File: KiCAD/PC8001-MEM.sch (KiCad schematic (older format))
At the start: 37 parts, among them J1 PC-8001 ext BUS, U1 74LS32, U10 628128, U2 74LS138, U3 ULN2003A, U4 74LS138, U5 74LS175, U6 74LS32, U7 74LS541, U8 74LS273, U9 74LS541

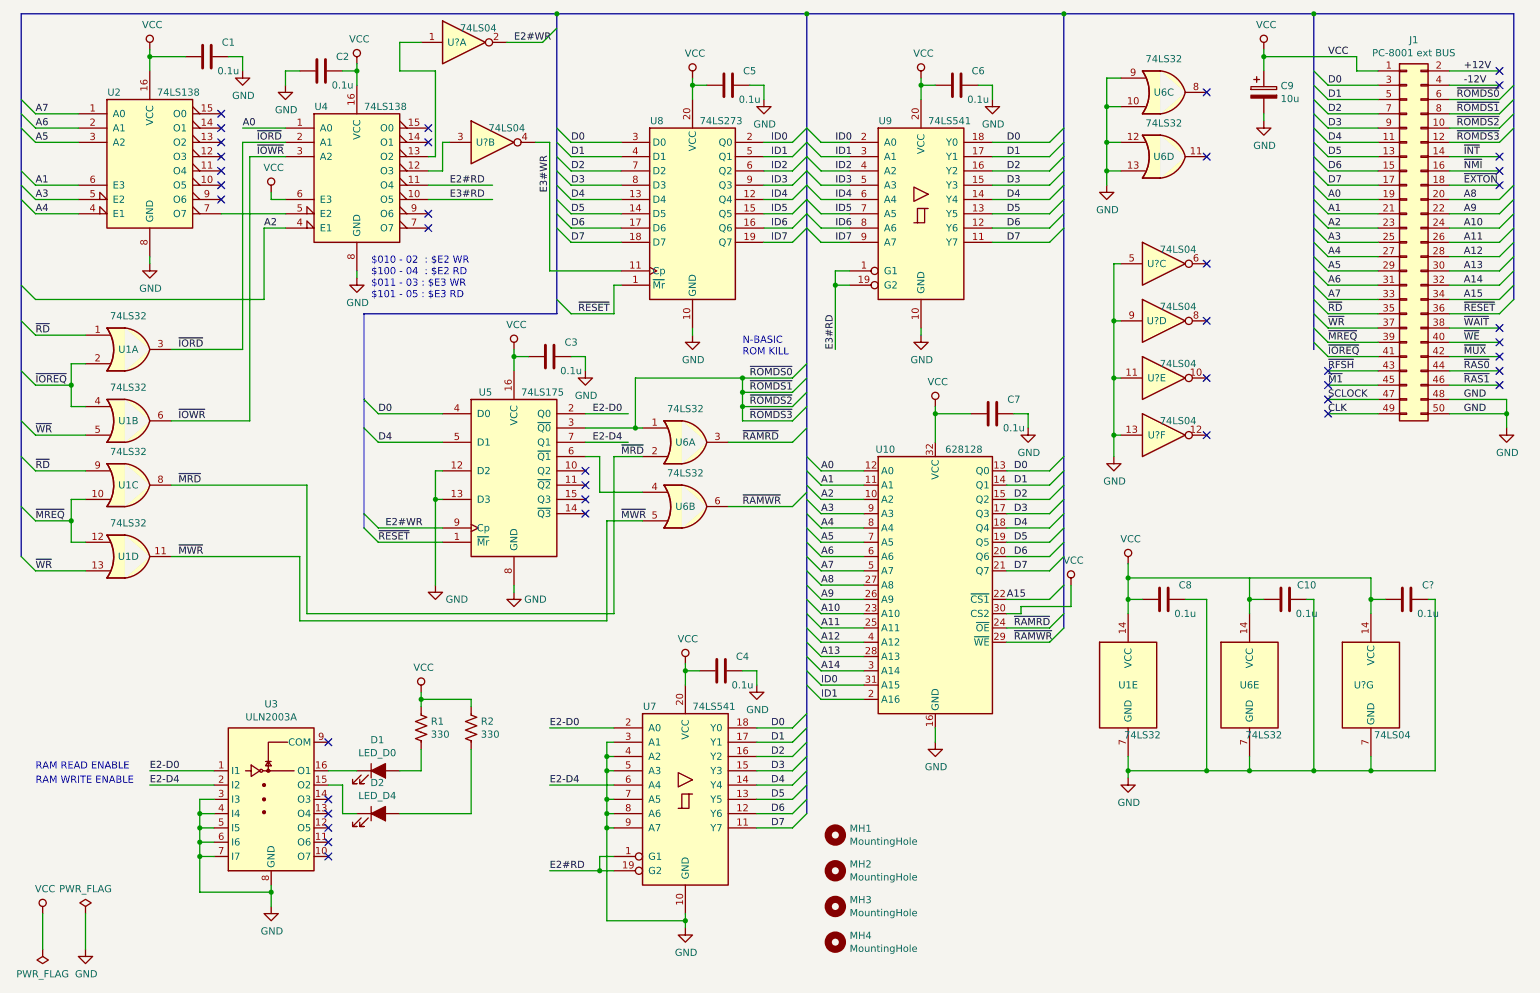
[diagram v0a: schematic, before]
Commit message: Revert "LS273、LS175のCp信号の部分の間違い訂正"
This reverts commit dc92f6c23538d2a9134d8bc83470156b4a3e76cd.
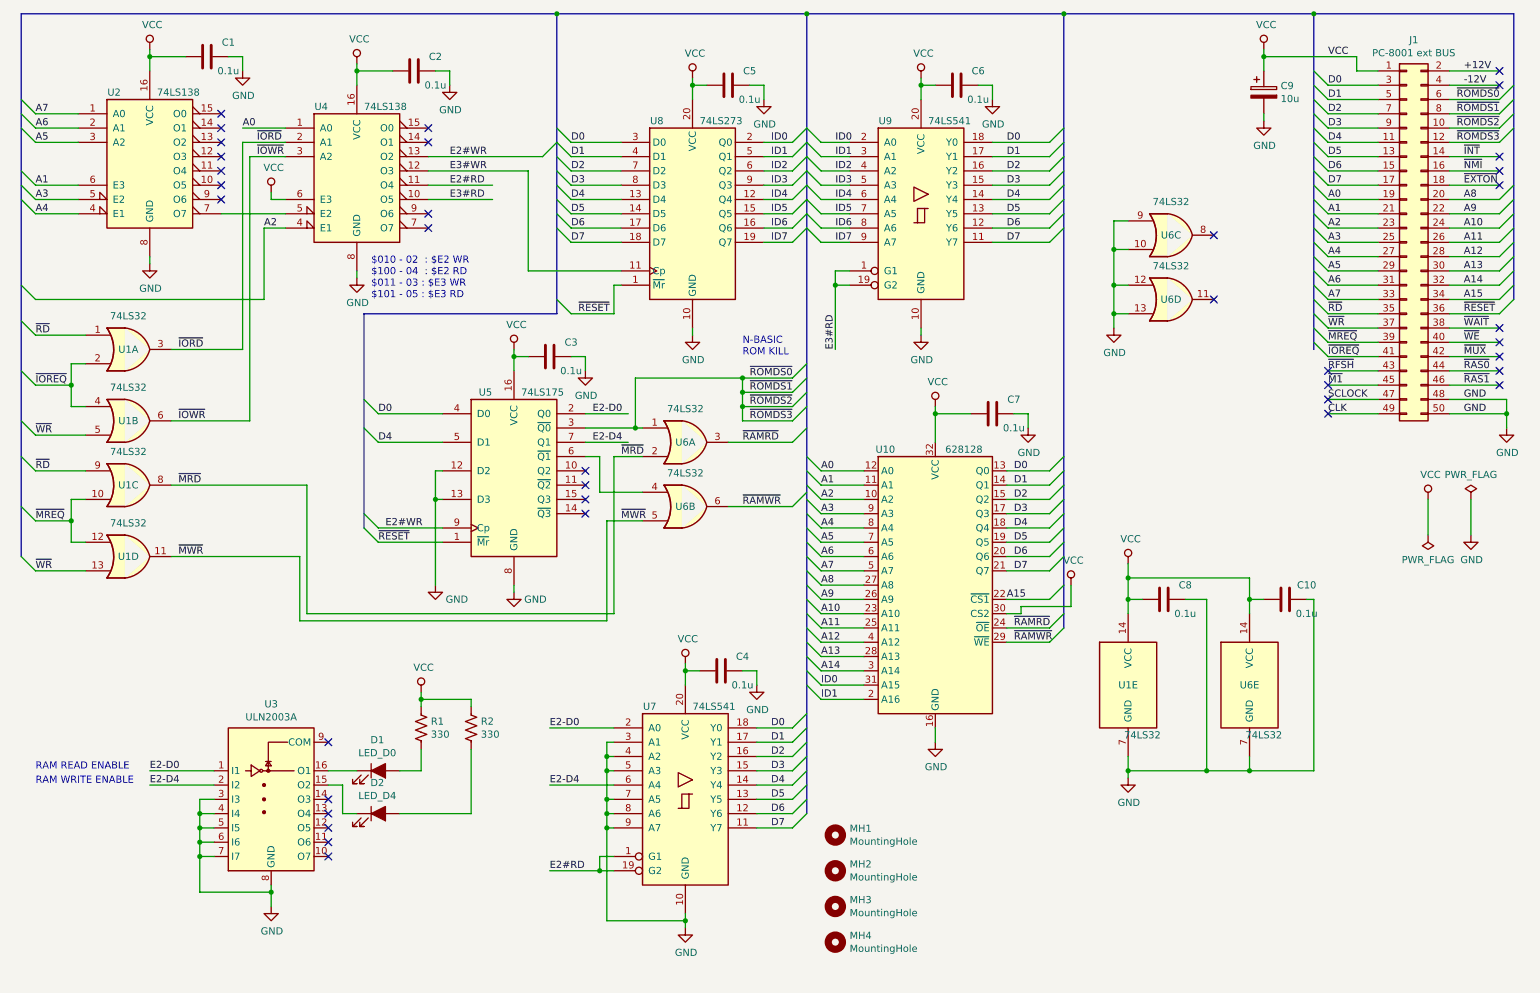
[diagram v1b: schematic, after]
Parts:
- removed C?: 0.1u, Capacitor_THT:C_Disc_D3.0mm_W1.6mm_P2.50mm, symbol Device:C
- removed U? (x7): 74LS04, symbol 74xx:74LS04
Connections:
- net E2#WR: now also U4.13 (O2)
- net E3#WR: now also U4.12 (O3)
- net GND: now also C2.1; no longer C2.2
- net VCC: now also C2.2; no longer C2.1
- no-connect marks 41 -> 37
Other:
- moved on the sheet: C2, U6C, U6D

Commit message: LS273、LS175のCp信号の部分の間違い訂正
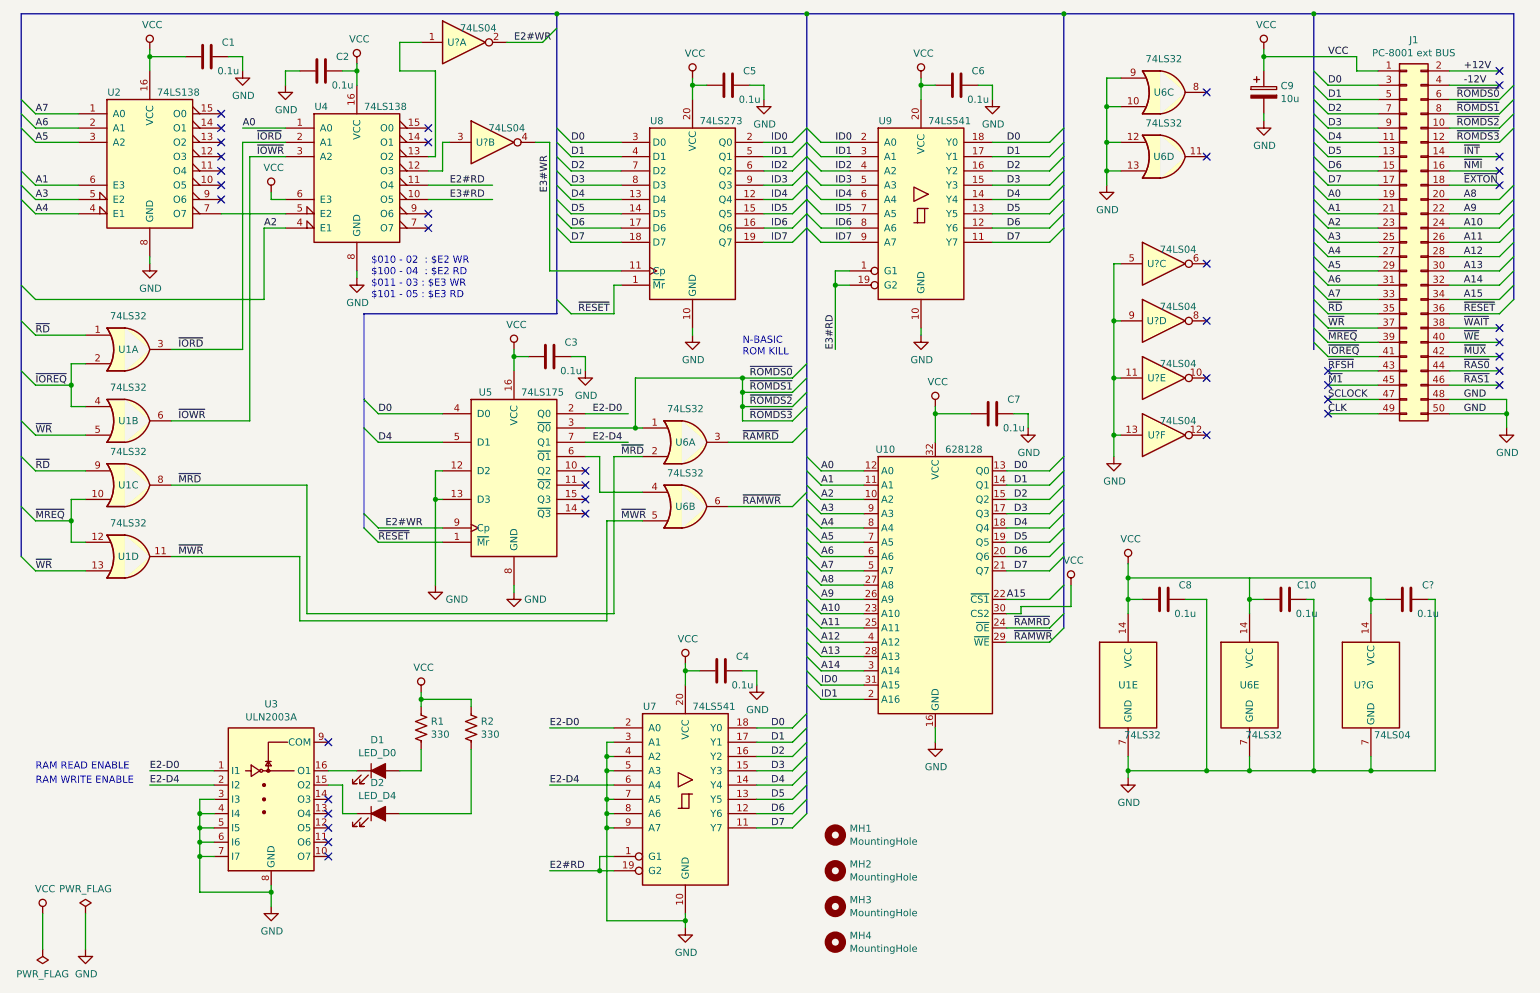
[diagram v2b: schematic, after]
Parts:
- added C?: 0.1u, Capacitor_THT:C_Disc_D3.0mm_W1.6mm_P2.50mm, symbol Device:C
- added U? (x7): 74LS04, symbol 74xx:74LS04
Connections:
- net E2#WR: now also U?.2; no longer U4.13 (O2)
- net E3#WR: now also U?.4; no longer U4.12 (O3)
- net GND: now also C2.2, C?.1, U?.11, U?.13, U?.5, U?.7 (GND), U?.9; no longer C2.1
- net VCC: now also C2.1, C?.2, U?.14 (VCC); no longer C2.2
- new net: U4.13 (O2), U?.1
- new net: U4.12 (O3), U?.3
- no-connect marks 37 -> 41
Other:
- moved on the sheet: C2, U6C, U6D
